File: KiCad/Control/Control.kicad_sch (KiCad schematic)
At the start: 27 parts, among them J1 TO_BACKPLANE, J2 TO_ALU, J3 TO_MEMORY, J4 TO_REGISTERS, J5 TO_MULDIV, J6 Conn_01x01, J7 Conn_01x01, J8 Conn_01x01, U10 74HCT32, U2 74HCT04, U22 74HCT32, U29 74HCT32, U9 74HCT08

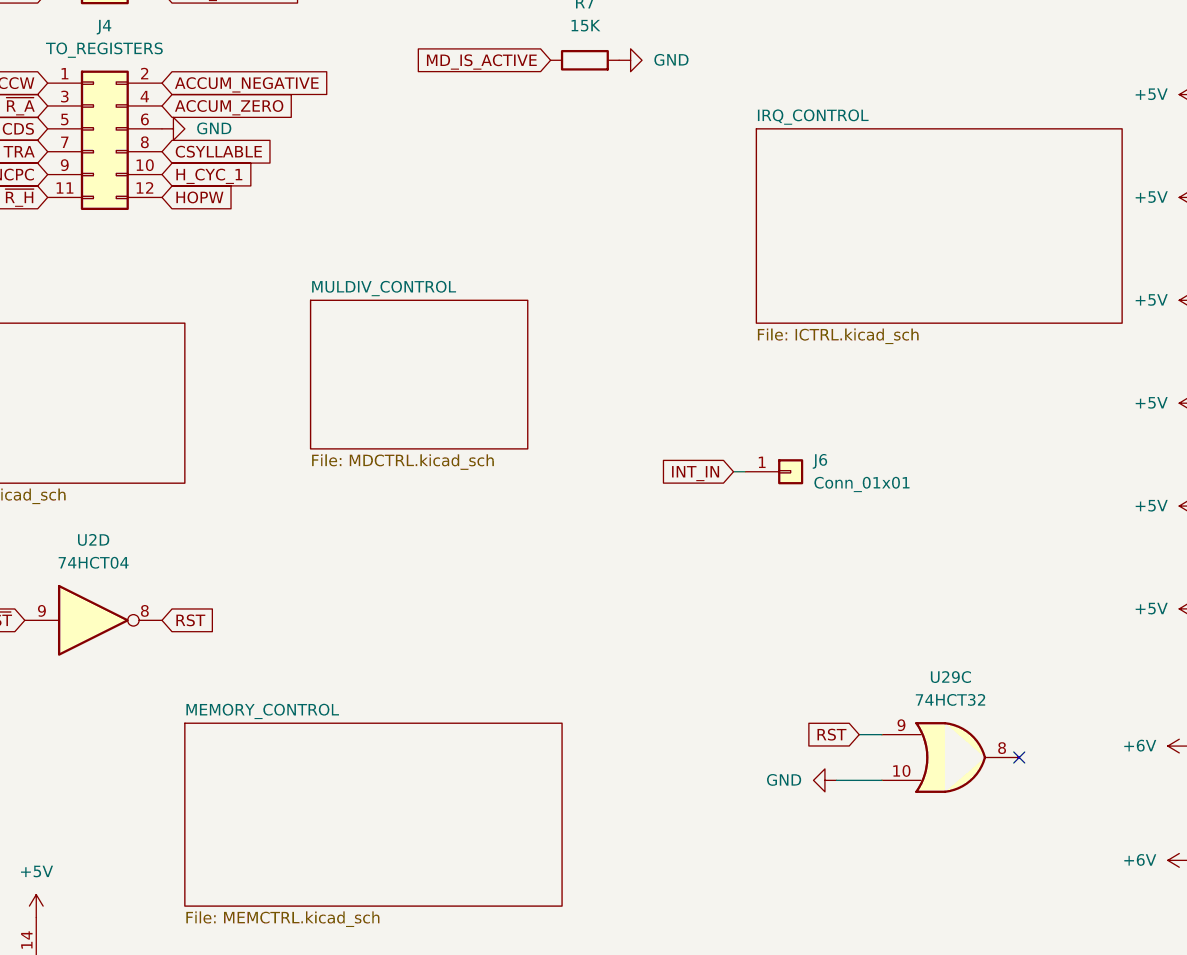
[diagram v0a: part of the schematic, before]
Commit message: Update schematics with fixes.
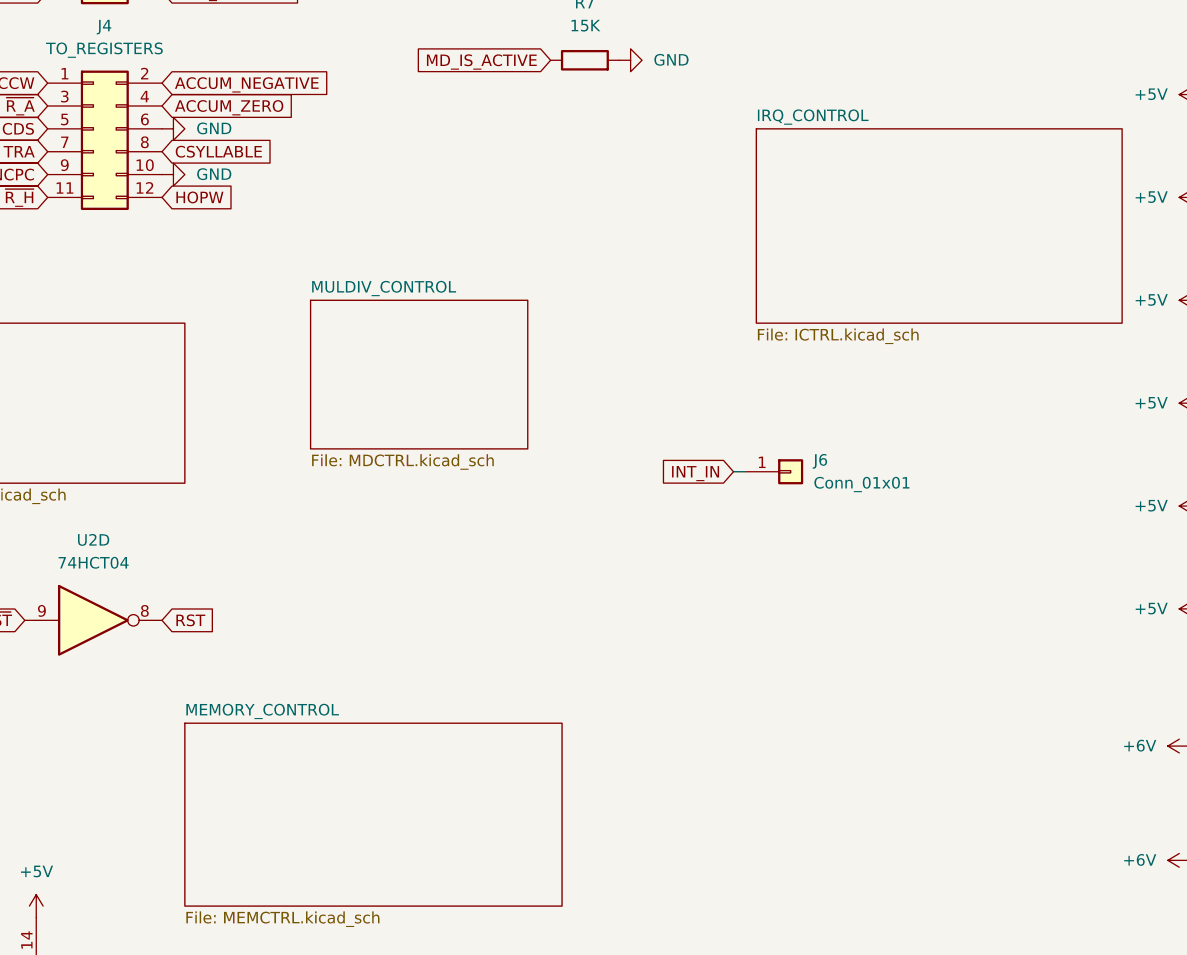
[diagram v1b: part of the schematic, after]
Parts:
- removed unit 3 of U29
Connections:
- net H_CYC_1 is gone; now on net GND: J4.10 (Pin_10)
- no-connect marks 1 -> 0
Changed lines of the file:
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@@
 		(color 0 0 0 0)
 	)
-	(no_connect
-		(at 184.15 125.73)
-	)
 	(wire
 		(pts
@@
 	(wire
 		(pts
-			(xy 163.83 128.27) (xy 168.91 128.27)
-		)
-		(stroke
-			(width 0)
-			(type default)
-		)
-	)
-	(wire
-		(pts
-			(xy 166.37 123.19) (xy 168.91 123.19)
-		)
-		(stroke
-			(width 0)
-			(type default)
-		)
-	)
-	(wire
-		(pts
 			(xy 44.45 53.34) (xy 43.18 53.34)
 		)
@@
 		)
 	)
-	(global_label "RST"
-		(shape input)
-		(at 166.37 123.19 180)
-		(fields_autoplaced yes)
-		(effects
-			(font
-				(size 1.27 1.27)
-			)
-			(justify right)
-		)
-		(property "Intersheetrefs" "${INTERSHEET_REFS}"
-			(at 159.9377 123.19 0)
-			(effects
-				(font
-					(size 1.27 1.27)
-				)
-				(justify right)
-				(hide yes)
-			)
-		)
-	)
 	(global_label "IS_EXM_I"
 		(shape input)
@@
 		)
 	)
-	(global_label "H_CYC_1"
-		(shape input)
-		(at 88.9 60.96 0)
-		(fields_autoplaced yes)
-		(effects
-			(font
-				(size 1.27 1.27)
-			)
-			(justify left)
-		)
-		(property "Intersheetrefs" "${INTERSHEET_REFS}"
-			(at 99.989 60.96 0)
-			(effects
-				(font
-					(size 1.27 1.27)
-				)
-				(justify left)
-				(hide yes)
-			)
-		)
-	)
 	(global_label "I7"
 		(shape input)
@@
 	)
 	(symbol
-		(lib_id "74xx:74LS32")
-		(at 176.53 125.73 0)
-		(unit 3)
-		(exclude_from_sim no)
-		(in_bom yes)
-		(on_board yes)
-		(dnp no)
-		(fields_autoplaced yes)
-		(property "Reference" "U29"
-			(at 176.53 116.84 0)
-			(effects
-				(font
-					(size 1.27 1.27)
-				)
-			)
-		)
-		(property "Value" "74HCT32"
-			(at 176.53 119.38 0)
-			(effects
-				(font
-					(size 1.27 1.27)
-				)
-			)
-		)
-		(property "Footprint" "Package_SO:SO-14_3.9x8.65mm_P1.27mm"
-			(at 176.53 125.73 0)
-			(effects
-				(font
-					(size 1.27 1.27)
-				)
-				(hide yes)
-			)
-		)
-		(property "Datasheet" "http://www.ti.com/lit/gpn/sn74LS32"
-			(at 176.53 125.73 0)
-			(effects
-				(font
-					(size 1.27 1.27)
-				)
-				(hide yes)
-			)
-		)
-		(property "Description" "Quad 2-input OR"
-			(at 176.53 125.73 0)
-			(effects
-				(font
-					(size 1.27 1.27)
-				)
-				(hide yes)
-			)
-		)
-		(property "VerilogCode" "ttl_74hct32 U29(_1, _2, _3, _4, _5, _6, _9, _10, _8, _12, _13, _11);"
-			(at 176.53 125.73 0)
-			(effects
-				(font
-					(size 1.27 1.27)
-				)
-				(hide yes)
-			)
-		)
-		(pin "10"
-		)
-		(pin "5"
-		)
-		(pin "3"
-		)
-		(pin "6"
-		)
-		(pin "9"
-		)
-		(pin "7"
-		)
-		(pin "4"
-		)
-		(pin "12"
-		)
-		(pin "11"
-		)
-		(pin "8"
-		)
-		(pin "1"
-		)
-		(pin "14"
-		)
-		(pin "13"
-		)
-		(pin "2"
-		)
-		(instances
-			(project ""
-				(path "/d9911e88-3002-43fe-906c-efbbcc56ef85"
-					(reference "U29")
-					(unit 3)
-				)
-			)
-		)
-	)
-	(symbol
 		(lib_id "power:GND")
 		(at 27.94 53.34 270)
@@
 	)
 	(symbol
-		(lib_id "power:GND")
-		(at 163.83 128.27 270)
-		(unit 1)
-		(exclude_from_sim no)
-		(in_bom yes)
-		(on_board yes)
-		(dnp no)
-		(fields_autoplaced yes)
-		(property "Reference" "#PWR0140"
-			(at 157.48 128.27 0)
-			(effects
-				(font
-					(size 1.27 1.27)
-				)
-				(hide yes)
-			)
-		)
-		(property "Value" "GND"
-			(at 160.02 128.2699 90)
-			(effects
-				(font
-					(size 1.27 1.27)
-				)
-				(justify right)
-			)
-		)
-		(property "Footprint" ""
-			(at 163.83 128.27 0)
-			(effects
-				(font
-					(size 1.27 1.27)
-				)
-				(hide yes)
-			)
-		)
-		(property "Datasheet" ""
-			(at 163.83 128.27 0)
-			(effects
-				(font
-					(size 1.27 1.27)
-				)
-				(hide yes)
-			)
-		)
-		(property "Description" "Power symbol creates a global label with name \"GND\" , ground"
-			(at 163.83 128.27 0)
-			(effects
-				(font
-					(size 1.27 1.27)
-				)
-				(hide yes)
-			)
-		)
-		(pin "1"
-		)
-		(instances
-			(project "Control"
-				(path "/d9911e88-3002-43fe-906c-efbbcc56ef85"
-					(reference "#PWR0140")
-					(unit 1)
-				)
-			)
-		)
-	)
-	(symbol
 		(lib_id "Connector_Generic:Conn_02x06_Odd_Even")
 		(at 81.28 33.02 0)
@@
 					(unit 1)
 				)
+			)
+		)
+	)
+	(symbol
+		(lib_id "power:GND")
+		(at 88.9 60.96 90)
+		(unit 1)
+		(exclude_from_sim no)
+		(in_bom yes)
+		(on_board yes)
+		(dnp no)
+		(fields_autoplaced yes)
+		(property "Reference" "#PWR0140"
+			(at 95.25 60.96 0)
+			(effects
+				(font
+					(size 1.27 1.27)
+				)
+				(hide yes)
+			)
+		)
+		(property "Value" "GND"
+			(at 92.71 60.9599 90)
+			(effects
+				(font
+					(size 1.27 1.27)
+				)
+				(justify right)
+			)
+		)
+		(property "Footprint" ""
+			(at 88.9 60.96 0)
+			(effects
+				(font
+					(size 1.27 1.27)
+				)
+				(hide yes)
+			)
+		)
+		(property "Datasheet" ""
+			(at 88.9 60.96 0)
+			(effects
+				(font
+					(size 1.27 1.27)
+				)
+				(hide yes)
+			)
+		)
+		(property "Description" "Power symbol creates a global label with name \"GND\" , ground"
+			(at 88.9 60.96 0)
+			(effects
+				(font
+					(size 1.27 1.27)
+				)
+				(hide yes)
+			)
+		)
+		(pin "1"
+		)
+		(instances
+			(project "Control"
+				(path "/d9911e88-3002-43fe-906c-efbbcc56ef85"
+					(reference "#PWR0140")
+					(unit 1)
+				)
